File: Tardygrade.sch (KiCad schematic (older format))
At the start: 25 parts, among them J1 Conn_01x03, J2 Conn_01x03, J3 Conn_01x03, J4 Conn_01x03, Q1 FET, Q2 FET, U1 MCP1642B, U2 HUZZAH32, U3 Tinypico, U4 HallSwitch, U5 HallSwitch, U6 HallSwitch, U7 HallSwitch, X1 XpansionHeader

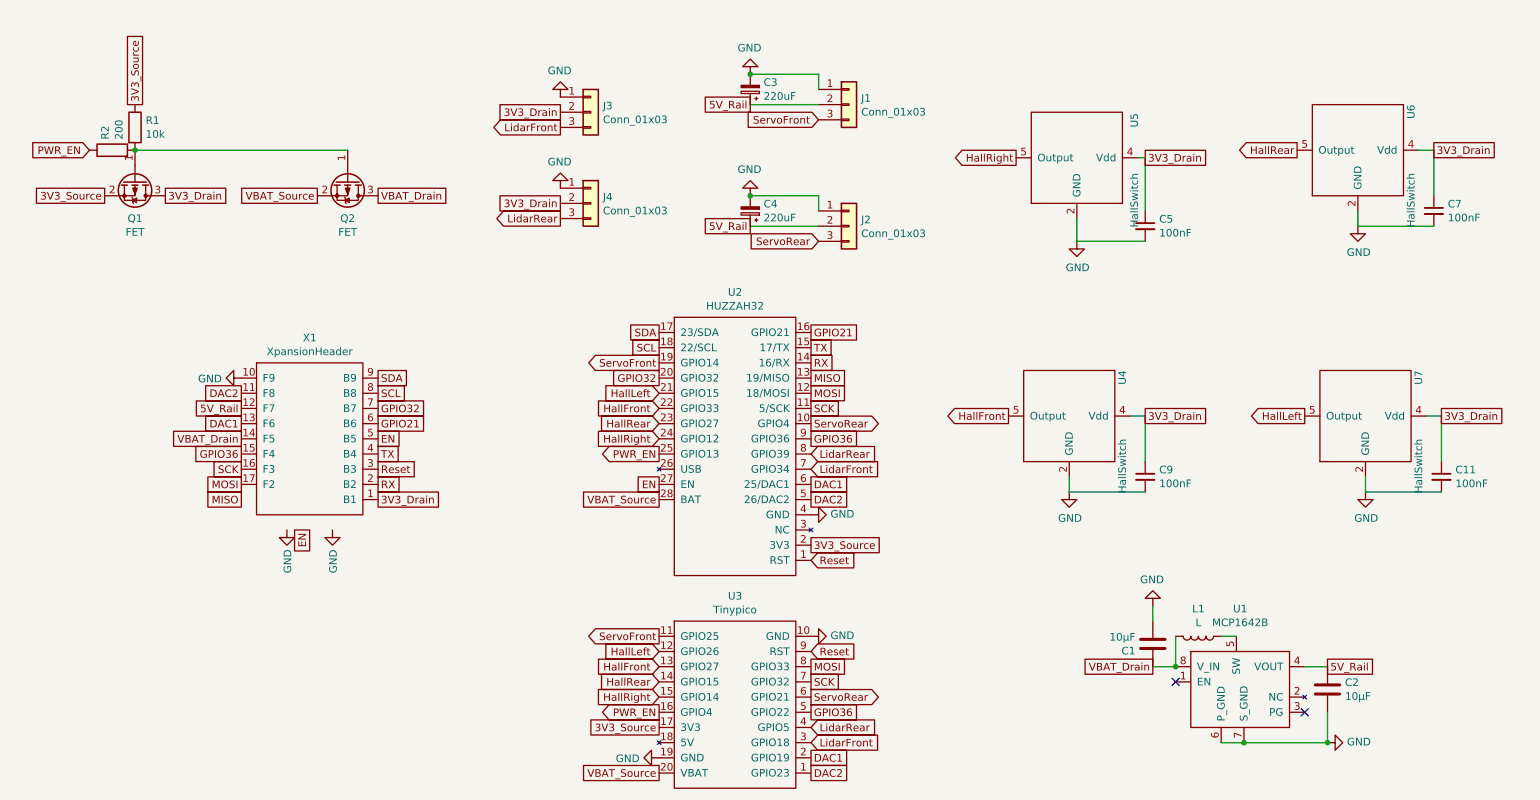
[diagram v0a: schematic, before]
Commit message: v0.4 update
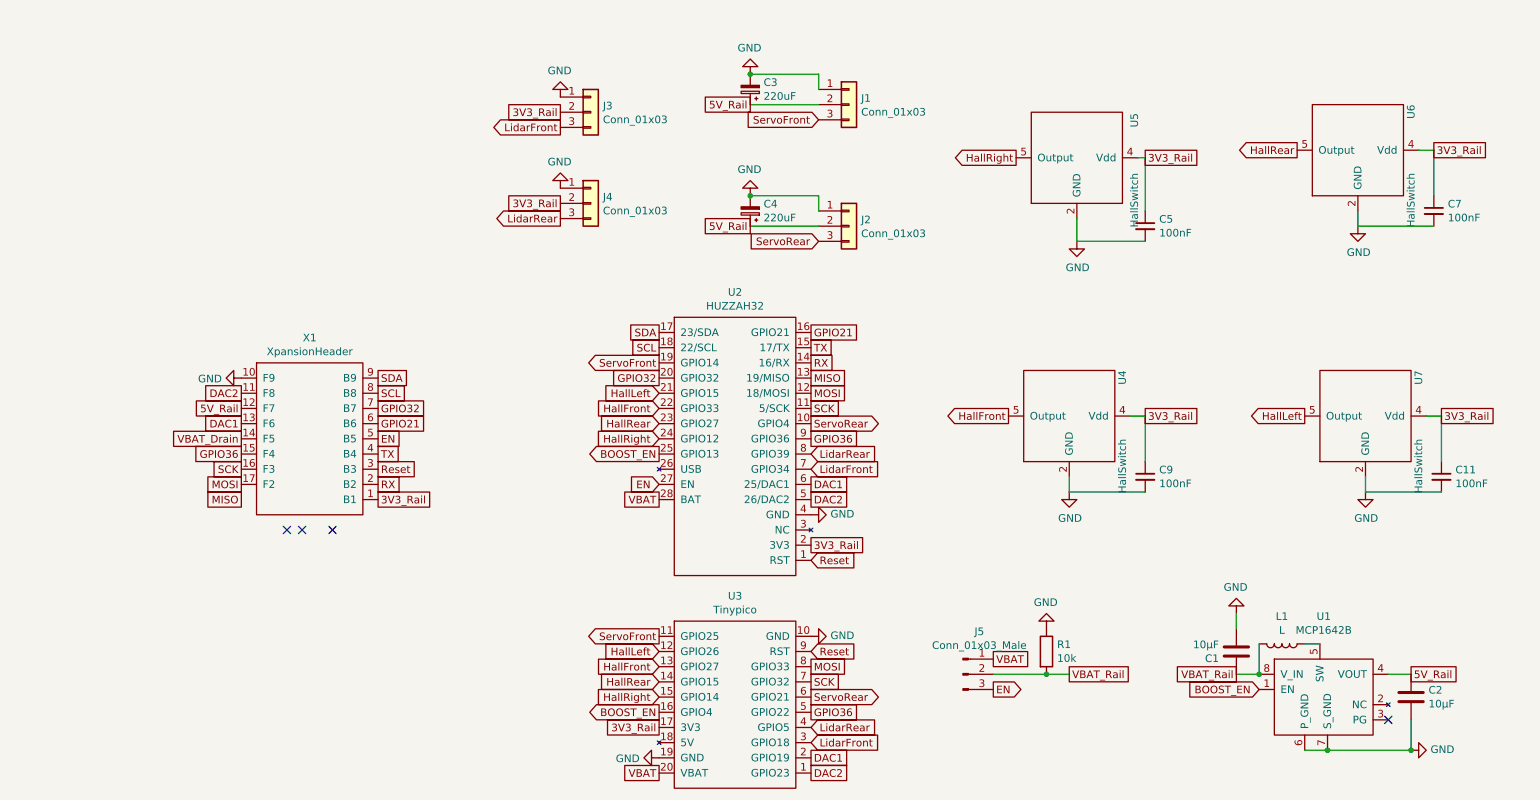
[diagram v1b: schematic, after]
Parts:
- removed Q1, Q2: FET, 222footprints:SOT-23_Handsolder, symbol Transistor_FET:AO3401A
- removed R2: 200, Resistor_SMD:R_0603_1608Metric_Pad0.98x0.95mm_HandSolder, symbol Device:R
- added J5: Conn_01x03_Male, Connector_PinHeader_2.54mm:PinHeader_1x03_P2.54mm_Vertical, symbol Connector:Conn_01x03_Male
- R1: footprint Resistor_SMD:R_0603_1608Metric_Pad0.98x0.95mm_HandSolder -> Resistor_SMD:R_0201_0603Metric_Pad0.64x0.40mm_HandSolder
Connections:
- net PWR_EN is gone; now on net BOOST_EN: U2.25 (GPIO13), U3.16 (GPIO4)
- net EN: now also J5.3 (Pin_3)
- net GND: now also R1.1
- net VBAT_Drain: no longer C1.1, L1.2, U1.8 (V_IN)
- net BOOST_EN: now reaches U1.1 (EN)
- net VBAT_Rail: now reaches R1.2
- net VBAT_Rail: now also C1.1, L1.2, U1.8 (V_IN), J5.2 (Pin_2)
- net 3V3_Drain renamed 3V3_Rail
- net 3V3_Rail: now also U2.2 (3V3), U3.17 (3V3)
- removed net 3V3_Source: R1.1, U2.2 (3V3), U3.17 (3V3)
- net VBAT_Source renamed VBAT
- net VBAT: now also J5.1 (Pin_1)
- no-connect marks 2 -> 4
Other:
- moved on the sheet: C1, C2, L1, U1

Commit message: v.04 update3
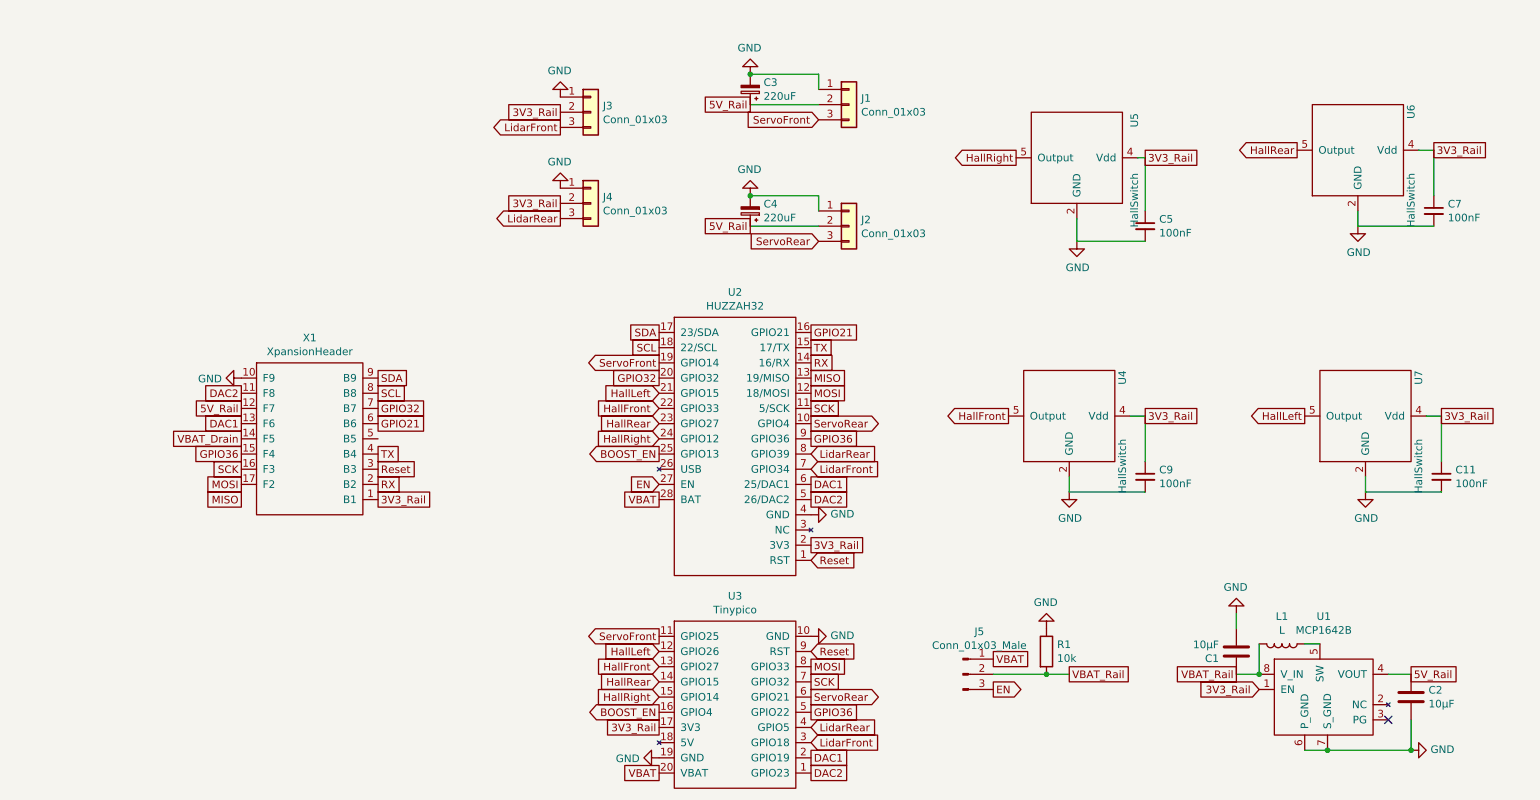
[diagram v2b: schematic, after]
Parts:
- R1: footprint Resistor_SMD:R_0201_0603Metric_Pad0.64x0.40mm_HandSolder -> Resistor_SMD:R_0603_1608Metric_Pad0.98x0.95mm_HandSolder
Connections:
- net 3V3_Rail: now also U1.1 (EN)
- net BOOST_EN: no longer U1.1 (EN)
- net EN: no longer X1.5 (B5)
- no-connect marks 4 -> 1
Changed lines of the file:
@@
 Text GLabel 6500 4800 2    50   Input ~ 0
 Reset
-Text GLabel 3650 3400 2    50   UnSpc ~ 0
-EN
 Text GLabel 3650 3600 2    50   UnSpc ~ 0
 Reset
@@
 	6550 1800 6550 1900
 Connection ~ 6100 1800
-NoConn ~ 3150 4000
-NoConn ~ 3350 4000
-NoConn ~ 3050 4000
 Text GLabel 9450 5050 0    50   Input ~ 0
-BOOST_EN
+3V3_Rail
 $Comp
 L Connector:Conn_01x03_Male J5
@@
 	9300 4550 9300 4650
 $Comp
-L power:GND #PWR?
+L power:GND #PWR0115
 U 1 1 617929C8
 P 8050 4650
-F 0 "#PWR?" H 8050 4400 50  0001 C CNN
+F 0 "#PWR0115" H 8050 4400 50  0001 C CNN
 F 1 "GND" H 8055 4477 50  0000 C CNN
 F 2 "" H 8050 4650 50  0001 C CNN
@@
 F 0 "R1" H 8120 4846 50  0000 L CNN
 F 1 "10k" H 8120 4755 50  0000 L CNN
-F 2 "Resistor_SMD:R_0201_0603Metric_Pad0.64x0.40mm_HandSolder" V 7980 4800 50  0001 C CNN
+F 2 "Resistor_SMD:R_0603_1608Metric_Pad0.98x0.95mm_HandSolder" V 7980 4800 50  0001 C CNN
 F 3 "~" H 8050 4800 50  0001 C CNN
 	1    8050 4800

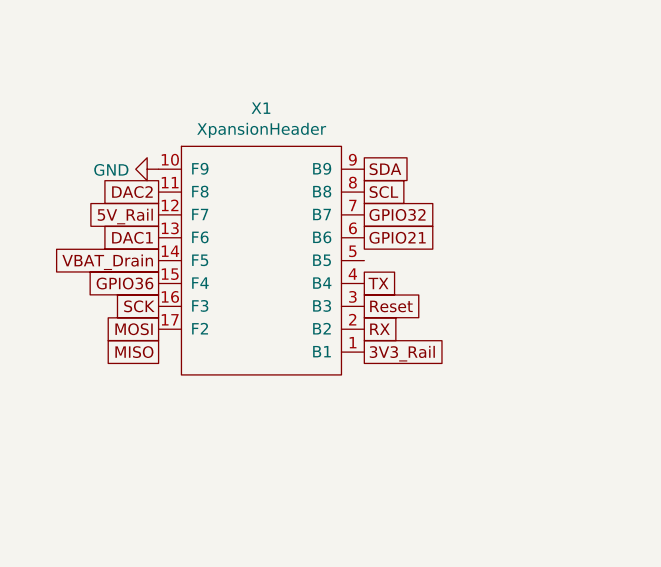
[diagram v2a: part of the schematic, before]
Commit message: v0.4 update 4
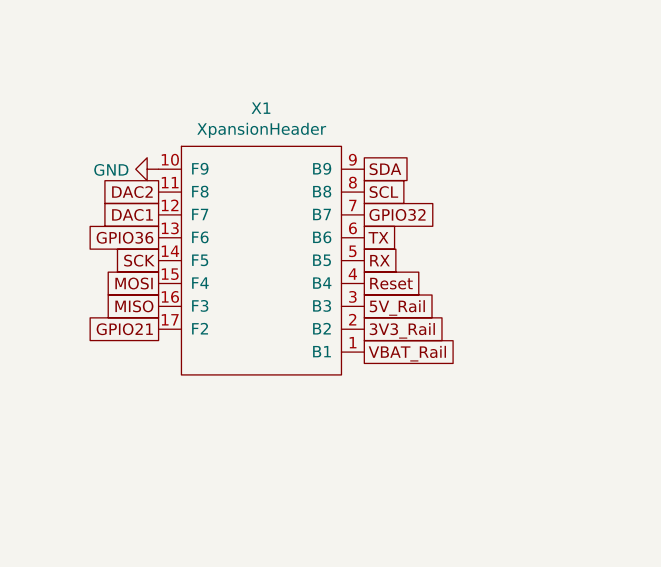
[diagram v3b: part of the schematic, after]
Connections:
- net VBAT_Drain is gone; now on net SCK: X1.14 (F5)
- net 3V3_Rail: now also X1.2 (B2); no longer X1.1 (B1)
- net 5V_Rail: now also X1.3 (B3); no longer X1.12 (F7)
- net DAC1: now also X1.12 (F7); no longer X1.13 (F6)
- net GPIO21: now also X1.17 (F2); no longer X1.6 (B6)
- net GPIO36: now also X1.13 (F6); no longer X1.15 (F4)
- net MISO: now also X1.16 (F3)
- net MOSI: now also X1.15 (F4); no longer X1.17 (F2)
- net RX: now also X1.5 (B5); no longer X1.2 (B2)
- net Reset: now also X1.4 (B4); no longer X1.3 (B3)
- net SCK: no longer X1.16 (F3)
- net TX: now also X1.6 (B6); no longer X1.4 (B4)
- net VBAT_Rail: now also X1.1 (B1)
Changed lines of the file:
@@
 	1    0    0    -1
 $EndComp
-Text GLabel 3650 3800 2    50   UnSpc ~ 0
+Text GLabel 3650 3700 2    50   UnSpc ~ 0
 3V3_Rail
 $Comp
@@
 	0    1    1    0
 $EndComp
-Text GLabel 2750 3200 0    50   UnSpc ~ 0
+Text GLabel 3650 3600 2    50   UnSpc ~ 0
 5V_Rail
 Text GLabel 6500 3800 2    50   UnSpc ~ 0
@@
 Text GLabel 2750 3100 0    50   UnSpc ~ 0
 DAC2
-Text GLabel 2750 3300 0    50   UnSpc ~ 0
+Text GLabel 2750 3200 0    50   UnSpc ~ 0
 DAC1
-Text GLabel 2750 3400 0    50   UnSpc ~ 0
-VBAT_Drain
+Text GLabel 3650 3800 2    50   UnSpc ~ 0
+VBAT_Rail
 Text GLabel 6500 3400 2    50   UnSpc ~ 0
 GPIO36
@@
 Text GLabel 6500 2700 2    50   UnSpc ~ 0
 GPIO21
+Text GLabel 2750 3300 0    50   UnSpc ~ 0
+GPIO36
+Text GLabel 2750 3400 0    50   UnSpc ~ 0
+SCK
 Text GLabel 2750 3500 0    50   UnSpc ~ 0
-GPIO36
-Text GLabel 2750 3600 0    50   UnSpc ~ 0
-SCK
-Text GLabel 2750 3700 0    50   UnSpc ~ 0
 MOSI
-Text GLabel 2750 3800 0    50   UnSpc ~ 0
-MISO
 Text GLabel 5500 2700 0    50   UnSpc ~ 0
 SDA
@@
 Text GLabel 3650 3200 2    50   UnSpc ~ 0
 GPIO32
+Text GLabel 2750 3700 0    50   UnSpc ~ 0
+GPIO21
 Text GLabel 3650 3300 2    50   UnSpc ~ 0
-GPIO21
-Text GLabel 3650 3500 2    50   UnSpc ~ 0
 TX
-Text GLabel 3650 3700 2    50   UnSpc ~ 0
+Text GLabel 3650 3400 2    50   UnSpc ~ 0
 RX
 Text GLabel 6500 4800 2    50   Input ~ 0
 Reset
-Text GLabel 3650 3600 2    50   UnSpc ~ 0
+Text GLabel 3650 3500 2    50   UnSpc ~ 0
 Reset
 Text GLabel 6500 4900 2    50   UnSpc ~ 0
@@
 Text GLabel 9300 4950 0    50   UnSpc ~ 0
 VBAT_Rail
+Text GLabel 2750 3600 0    50   UnSpc ~ 0
+MISO
 $EndSCHEMATC

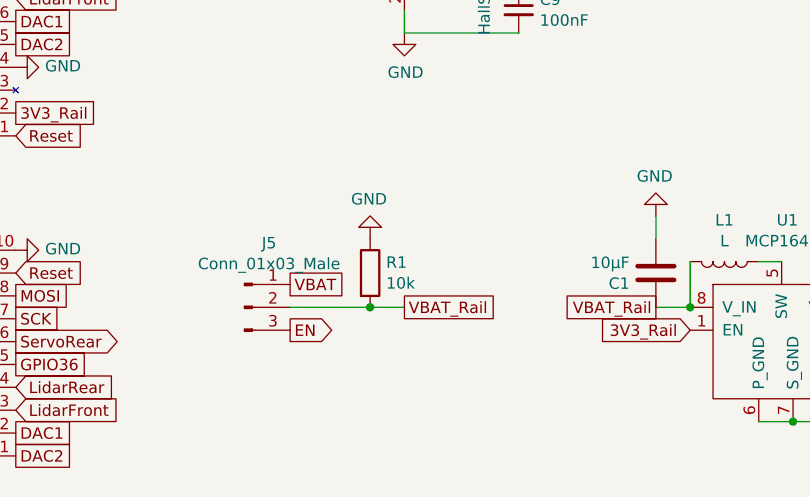
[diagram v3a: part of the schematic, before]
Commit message: v0.4 update 5
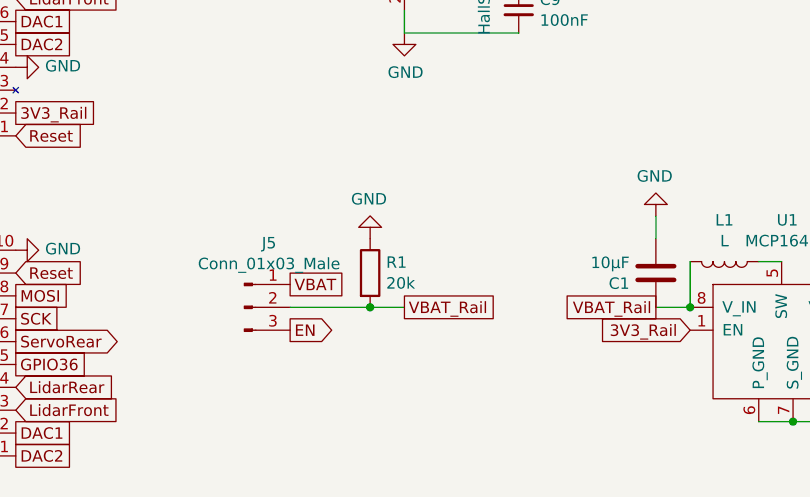
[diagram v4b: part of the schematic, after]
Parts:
- R1: value 10k -> 20k
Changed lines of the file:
@@
 P 8050 4800
 F 0 "R1" H 8120 4846 50  0000 L CNN
-F 1 "10k" H 8120 4755 50  0000 L CNN
+F 1 "20k" H 8120 4755 50  0000 L CNN
 F 2 "Resistor_SMD:R_0603_1608Metric_Pad0.98x0.95mm_HandSolder" V 7980 4800 50  0001 C CNN
 F 3 "~" H 8050 4800 50  0001 C CNN
